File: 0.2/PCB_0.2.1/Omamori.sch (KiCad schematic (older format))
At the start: 29 parts, among them J1 Conn_01x04_Female, U1 BQ25504, U2 TPS61222DCK, U3 ATtiny85, U4 TS-1233

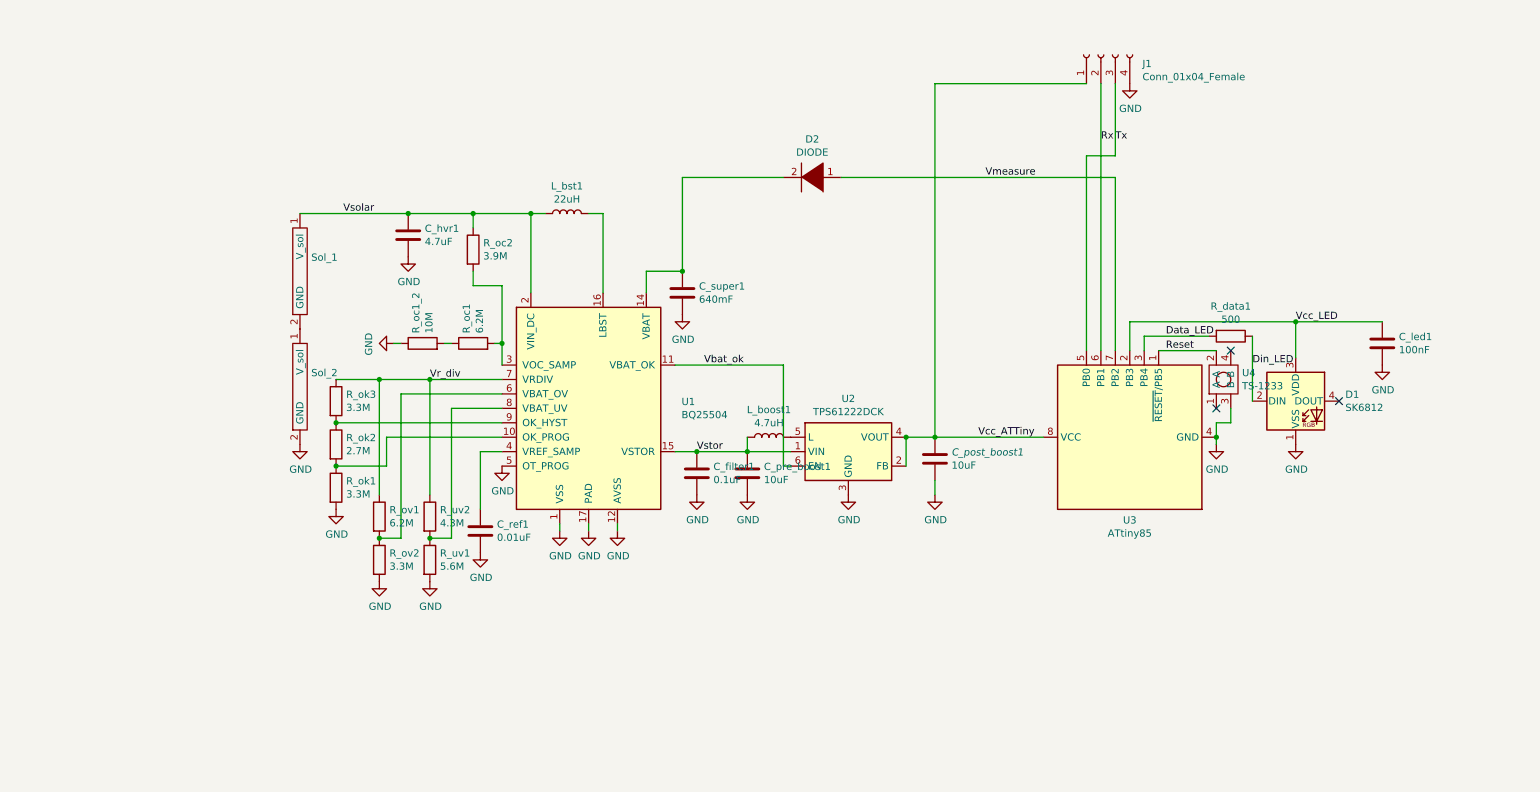
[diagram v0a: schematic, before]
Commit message: Updated 0.2.1 PCB design.
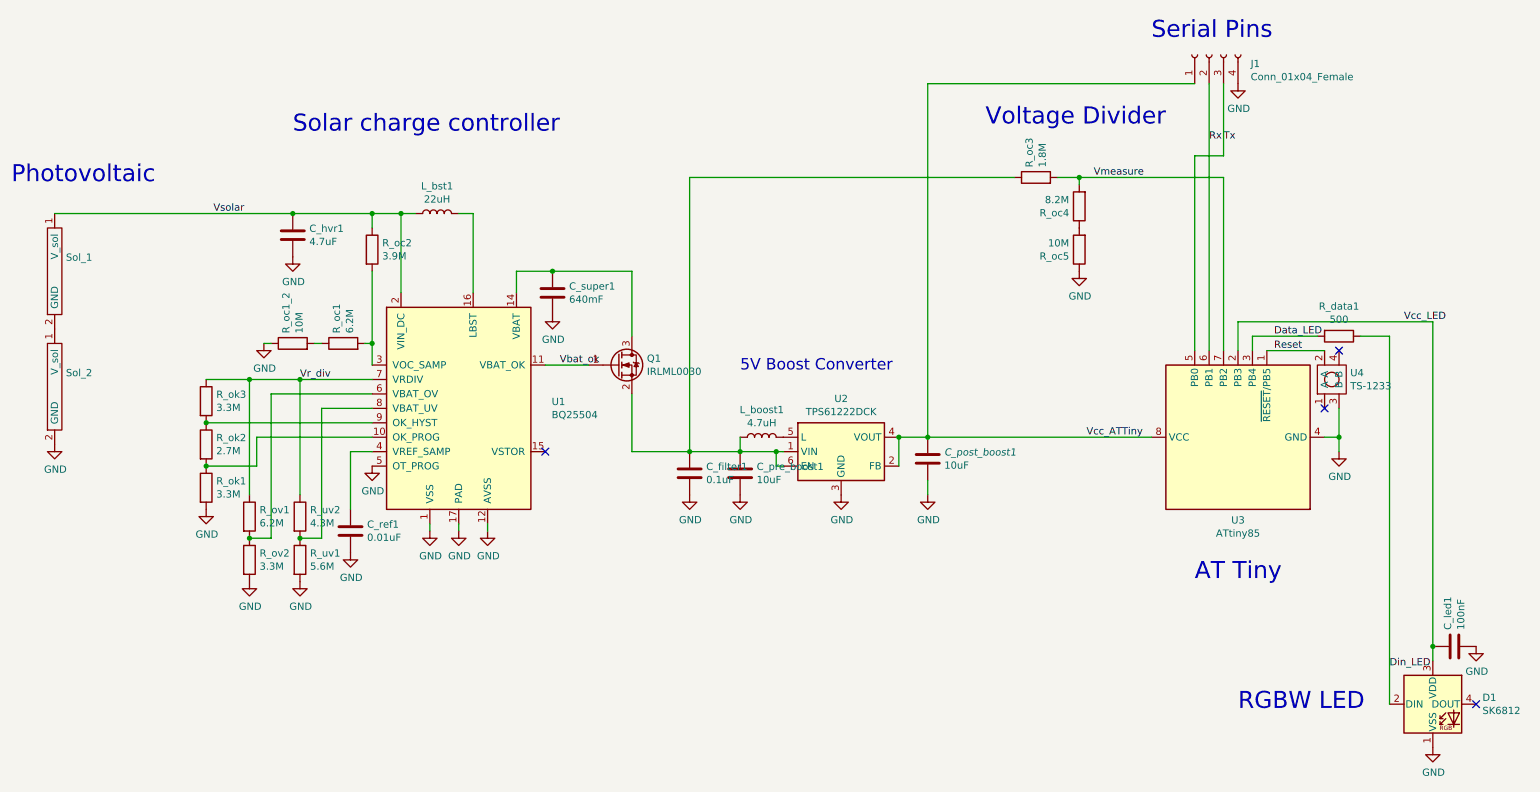
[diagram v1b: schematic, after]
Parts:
- removed D2: DIODE, Diode_SMD:D_SOD-323_HandSoldering, symbol pspice:DIODE
- added Q1: IRLML0030, Package_TO_SOT_SMD:SOT-23, symbol Transistor_FET:IRLML0030
- added R_oc3: 1.8M, Resistor_SMD:R_0603_1608Metric_Pad0.98x0.95mm_HandSolder, symbol Device:R
- added R_oc4: 8.2M, Resistor_SMD:R_0603_1608Metric_Pad0.98x0.95mm_HandSolder, symbol Device:R
- added R_oc5: 10M, Resistor_SMD:R_0603_1608Metric_Pad0.98x0.95mm_HandSolder, symbol Device:R
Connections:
- net GND: now also R_oc5.1
- net Vbat_ok: now also Q1.1 (G); no longer U2.6 (EN)
- net Vmeasure: now also R_oc3.2, R_oc4.2
- net at C_super1.1, U1.14 (VBAT): now also Q1.3 (D)
- net Vstor: no longer names the net of C_filter1.1, C_pre_boost1.1, L_boost1.1, U2.1 (VIN)
- net Vstor: now also U2.6 (EN), Q1.2 (S), R_oc3.1; no longer U1.15 (VSTOR)
- new net: R_oc4.1, R_oc5.2
- no-connect marks 3 -> 4
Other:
- note added: "5V Boost Converter\n"
- note added: "AT Tiny\n"
- note added: "Photovoltaic"
- note added: "RGBW LED"
- note added: "Serial Pins\n"
- note added: "Solar charge controller"
- note added: "Voltage Divider\n"
- moved on the sheet: C_filter1, C_hvr1, C_led1, C_post_boost1, C_pre_boost1, C_ref1, C_super1, D1, J1, L_boost1, L_bst1, R_data1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
